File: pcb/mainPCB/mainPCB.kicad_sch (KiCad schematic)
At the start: 8 parts, among them J1 Conn_01x30, J2 Conn_02x15_Counter_Clockwise, J3 Conn_01x04_Shielded_Backlight, J4 Conn_02x03_Odd_Even_Backlight, Q1 BC547, U1 ESP32-S3-DevKitC

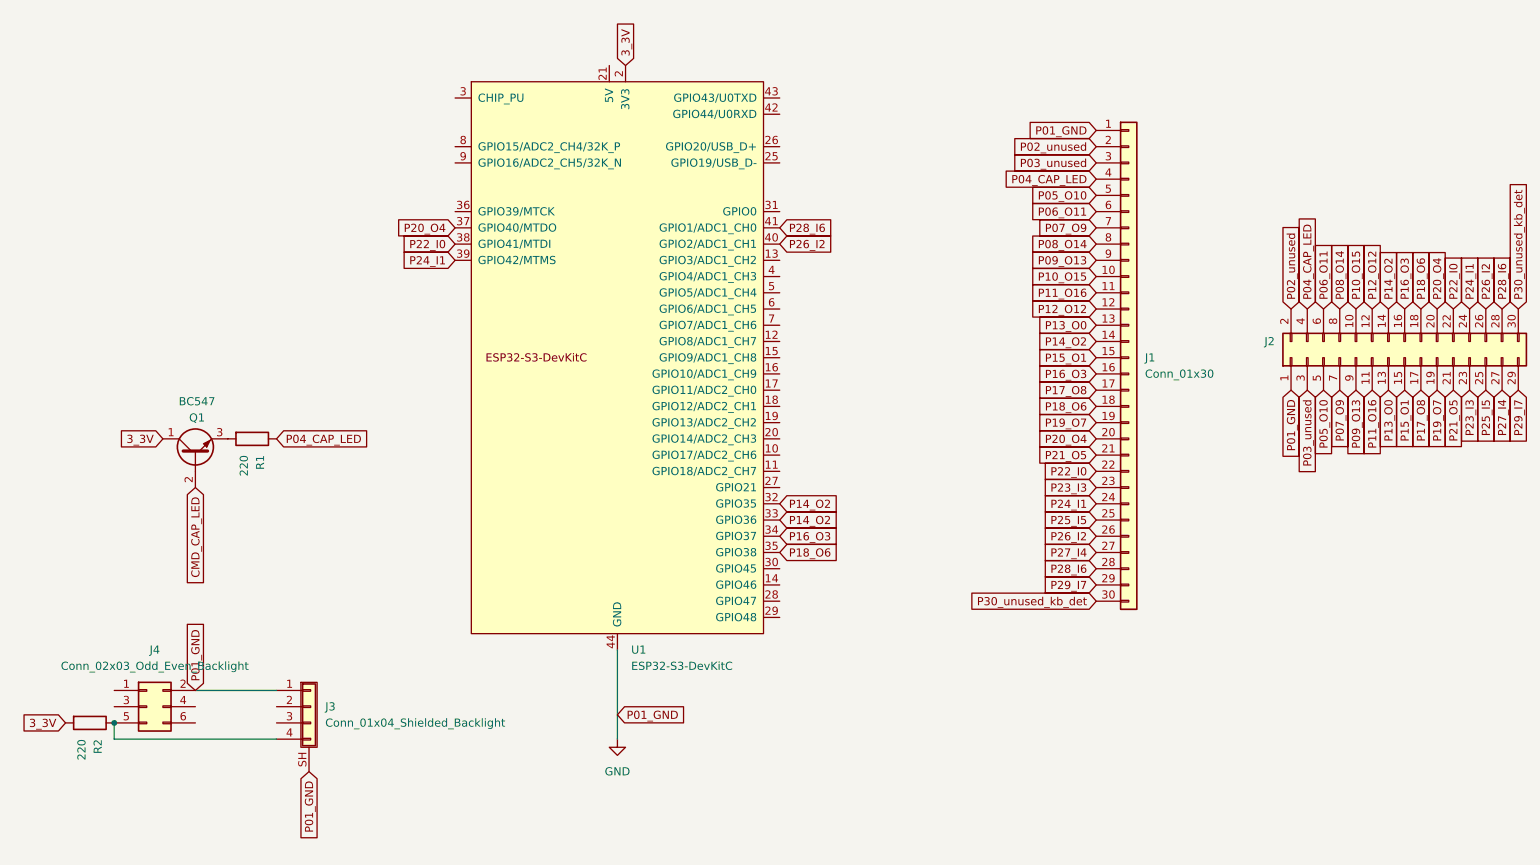
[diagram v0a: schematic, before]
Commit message: chore: more cables
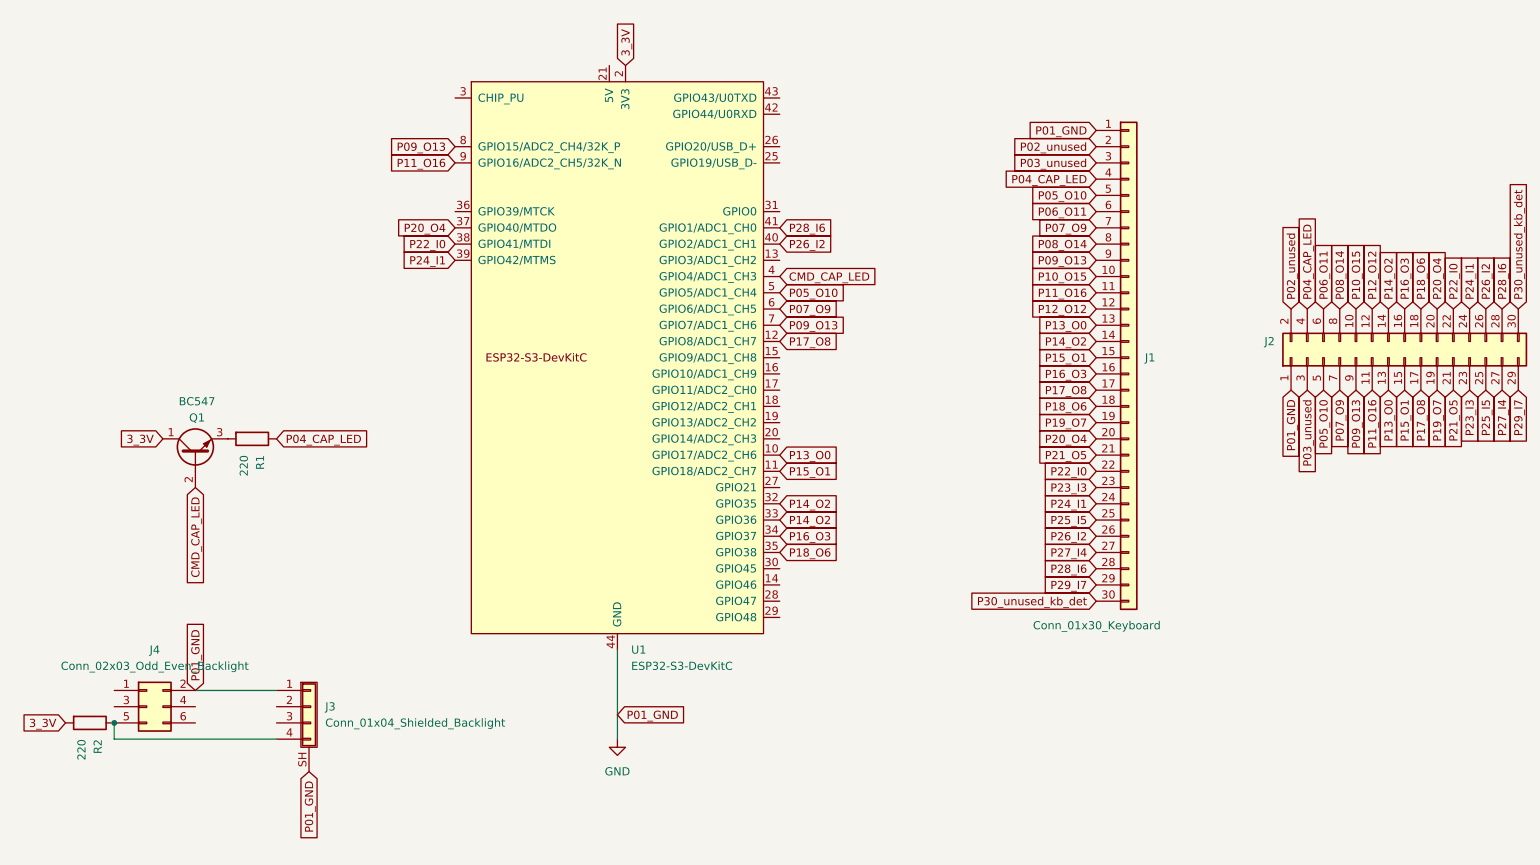
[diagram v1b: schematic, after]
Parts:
- J1: value Conn_01x30 -> Conn_01x30_Keyboard
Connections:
- net CMD_CAP_LED: now also U1.4 (GPIO4/ADC1_CH3)
- net P05_O10: now also U1.5 (GPIO5/ADC1_CH4)
- net P07_O9: now also U1.6 (GPIO6/ADC1_CH5)
- net P09_O13: now also U1.7 (GPIO7/ADC1_CH6), U1.8 (GPIO15/ADC2_CH4/32K_P)
- net P11_O16: now also U1.9 (GPIO16/ADC2_CH5/32K_N)
- net P13_O0: now also U1.10 (GPIO17/ADC2_CH6)
- net P15_O1: now also U1.11 (GPIO18/ADC2_CH7)
- net P17_O8: now also U1.12 (GPIO8/ADC1_CH7)
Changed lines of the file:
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@@
+		)
+	)
+	(global_label "P11_O16"
+		(shape input)
+		(at 104.14 67.31 180)
+		(fields_autoplaced yes)
+		(effects
+			(font
+				(size 1.27 1.27)
+			)
+			(justify right)
+		)
+		(property "Intersheetrefs" "${INTERSHEET_REFS}"
+			(at 92.7487 67.31 0)
+			(effects
+				(font
+					(size 1.27 1.27)
+				)
+				(justify right)
+				(hide yes)
+			)
 		)
 	)
@@
 		)
 	)
+	(global_label "CMD_CAP_LED"
+		(shape input)
+		(at 154.94 85.09 0)
+		(fields_autoplaced yes)
+		(effects
+			(font
+				(size 1.27 1.27)
+			)
+			(justify left)
+		)
+		(property "Intersheetrefs" "${INTERSHEET_REFS}"
+			(at 170.9275 85.09 0)
+			(effects
+				(font
+					(size 1.27 1.27)
+				)
+				(justify left)
+				(hide yes)
+			)
+		)
+	)
 	(global_label "P02_unused"
 		(shape input)
@@
 	(global_label "P07_O9"
 		(shape input)
+		(at 154.94 90.17 0)
+		(fields_autoplaced yes)
+		(effects
+			(font
+				(size 1.27 1.27)
+			)
+			(justify left)
+		)
+		(property "Intersheetrefs" "${INTERSHEET_REFS}"
+			(at 165.1218 90.17 0)
+			(effects
+				(font
+					(size 1.27 1.27)
+				)
+				(justify left)
+				(hide yes)
+			)
+		)
+	)
+	(global_label "P07_O9"
+		(shape input)
 		(at 242.57 102.87 270)
 		(fields_autoplaced yes)
@@
 		)
 	)
+	(global_label "P13_O0"
+		(shape input)
+		(at 154.94 113.03 0)
+		(fields_autoplaced yes)
+		(effects
+			(font
+				(size 1.27 1.27)
+			)
+			(justify left)
+		)
+		(property "Intersheetrefs" "${INTERSHEET_REFS}"
+			(at 165.1218 113.03 0)
+			(effects
+				(font
+					(size 1.27 1.27)
+				)
+				(justify left)
+				(hide yes)
+			)
+		)
+	)
+	(global_label "P09_O13"
+		(shape input)
+		(at 104.14 64.77 180)
+		(fields_autoplaced yes)
+		(effects
+			(font
+				(size 1.27 1.27)
+			)
+			(justify right)
+		)
+		(property "Intersheetrefs" "${INTERSHEET_REFS}"
+			(at 92.7487 64.77 0)
+			(effects
+				(font
+					(size 1.27 1.27)
+				)
+				(justify right)
+				(hide yes)
+			)
+		)
+	)
 	(global_label "P26_I2"
 		(shape input)
@@
 		)
 	)
+	(global_label "P15_O1"
+		(shape input)
+		(at 154.94 115.57 0)
+		(fields_autoplaced yes)
+		(effects
+			(font
+				(size 1.27 1.27)
+			)
+			(justify left)
+		)
+		(property "Intersheetrefs" "${INTERSHEET_REFS}"
+			(at 165.1218 115.57 0)
+			(effects
+				(font
+					(size 1.27 1.27)
+				)
+				(justify left)
+				(hide yes)
+			)
+		)
+	)
 	(global_label "P09_O13"
 		(shape input)
@@
 		)
 	)
+	(global_label "P17_O8"
+		(shape input)
+		(at 154.94 95.25 0)
+		(fields_autoplaced yes)
+		(effects
+			(font
+				(size 1.27 1.27)
+			)
+			(justify left)
+		)
+		(property "Intersheetrefs" "${INTERSHEET_REFS}"
+			(at 165.1218 95.25 0)
+			(effects
+				(font
+					(size 1.27 1.27)
+				)
+				(justify left)
+				(hide yes)
+			)
+		)
+	)
+	(global_label "P05_O10"
+		(shape input)
+		(at 154.94 87.63 0)
+		(fields_autoplaced yes)
+		(effects
+			(font
+				(size 1.27 1.27)
+			)
+			(justify left)
+		)
+		(property "Intersheetrefs" "${INTERSHEET_REFS}"
+			(at 166.3313 87.63 0)
+			(effects
+				(font
+					(size 1.27 1.27)
+				)
+				(justify left)
+				(hide yes)
+			)
+		)
+	)
 	(global_label "P01_GND"
 		(shape input)
@@
 				)
 				(justify right)
+				(hide yes)
+			)
+		)
+	)
+	(global_label "P09_O13"
+		(shape input)
+		(at 154.94 92.71 0)
+		(fields_autoplaced yes)
+		(effects
+			(font
+				(size 1.27 1.27)
+			)
+			(justify left)
+		)
+		(property "Intersheetrefs" "${INTERSHEET_REFS}"
+			(at 166.3313 92.71 0)
+			(effects
+				(font
+					(size 1.27 1.27)
+				)
+				(justify left)
 				(hide yes)
 			)
@@
 		(on_board yes)
 		(dnp no)
-		(fields_autoplaced yes)
 		(property "Reference" "J1"
 			(at 212.09 97.7899 0)
@@
 			)
 		)
-		(property "Value" "Conn_01x30"
-			(at 212.09 100.3299 0)
-			(effects
-				(font
+		(property "Value" "Conn_01x30_Keyboard"
+			(at 194.564 139.7 0)
+			(effects
+				(font
